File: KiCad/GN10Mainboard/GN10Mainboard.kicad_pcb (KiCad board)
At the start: 4 copper layers, 80 x 60 mm, 129 parts, among them J1 XT30PW-M, J10 USB_C_Receptacle_USB2.0, J13 Conn_01x06, J14 Conn_01x06, J4 Conn_01x04, J5 Conn_01x06, J6 Conn_01x04, J7 Conn_01x04, J8 Conn_01x04, J9 RJ45_Bel_SI-60062-F, SW1 SW_Push, U1 TPS54560DDA, U10 BNO086, U11 FT231XS, U2 3.3V, U4 STM32G474RETx, U5 MCP2562-E-SN, U6 MCP2562-E-SN, U7 MCP2562-E-SN, U8 W5500, Y1 24MHz, Y3 25M, Y6 32.768kHz, Y7 32.768kHz

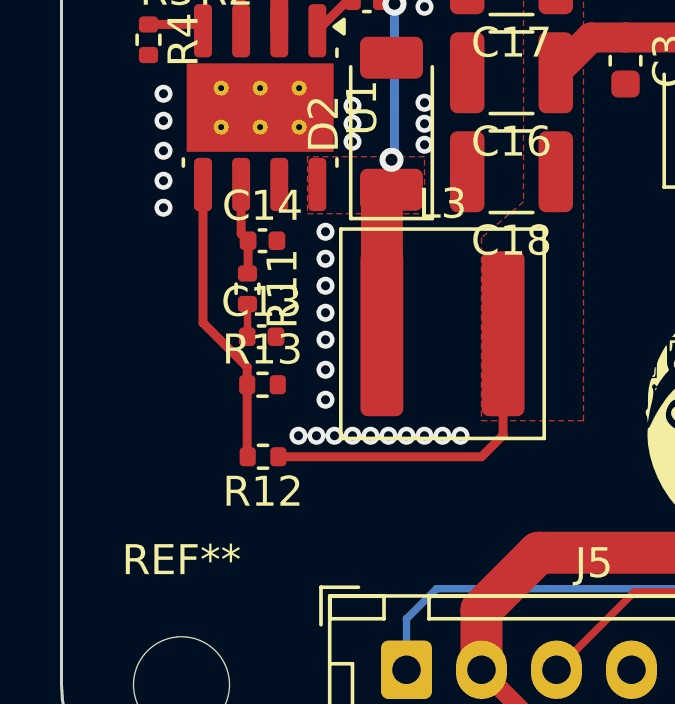
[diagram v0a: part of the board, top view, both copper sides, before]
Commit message: fix:feedback wire
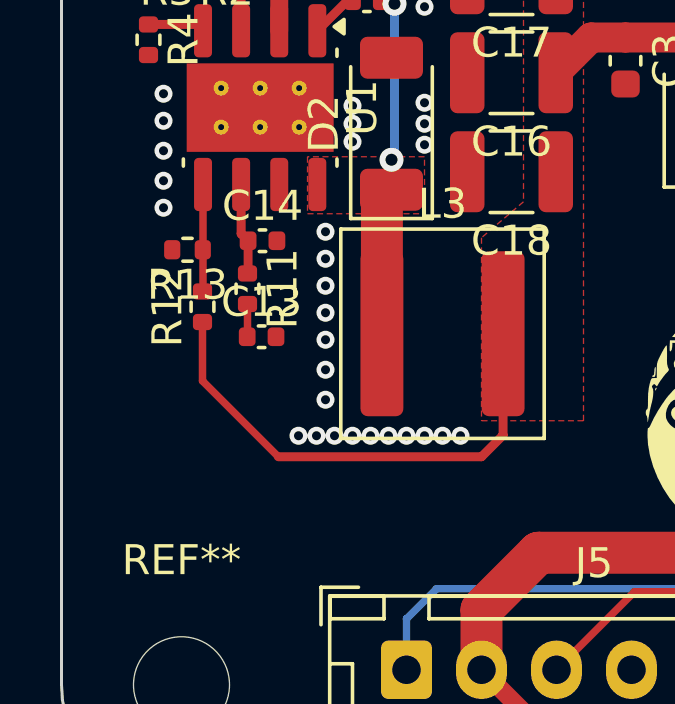
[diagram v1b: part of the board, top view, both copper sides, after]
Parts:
- moved R12 5.39 mm to (134.7, 133.4), turned to 90 degrees
- moved R13 5.15 mm to (134.2, 131.5), turned to 180 degrees
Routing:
- net Net-(U1-FB): track 9.69 -> 3.57 mm
- net +5V: track 98.4 -> 103.9 mm
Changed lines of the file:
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@@
 	(footprint "Resistor_SMD:R_0402_1005Metric"
 		(layer "F.Cu")
-		(at 136.7 136)
+		(at 134.2 131.5 180)
 		(descr "Resistor SMD 0402 (1005 Metric), square (rectangular) end terminal, IPC-7351 nominal, (Body size source: IPC-SM-782 page 72, https://www.pcb-3d.com/wordpress/wp-content/uploads/ipc-sm-782a_amendment_1_and_2.pdf), generated with kicad-footprint-generator")
 		(tags "resistor")
@@
 		(attr smd)
 		(fp_line
-			(start -0.153641 -0.38)
-			(end 0.153641 -0.38)
+			(start -0.153641 0.38)
+			(end 0.153641 0.38)
 			(stroke
 				(width 0.12)
@@
 		)
 		(fp_line
-			(start -0.153641 0.38)
-			(end 0.153641 0.38)
+			(start -0.153641 -0.38)
+			(end 0.153641 -0.38)
 			(stroke
 				(width 0.12)
@@
 		)
 		(fp_line
-			(start -0.93 -0.47)
-			(end 0.93 -0.47)
+			(start 0.93 0.47)
+			(end -0.93 0.47)
 			(stroke
 				(width 0.05)
@@
 		)
 		(fp_line
-			(start -0.93 0.47)
-			(end -0.93 -0.47)
+			(start 0.93 -0.47)
+			(end 0.93 0.47)
 			(stroke
 				(width 0.05)
@@
 		)
 		(fp_line
-			(start 0.93 -0.47)
-			(end 0.93 0.47)
+			(start -0.93 0.47)
+			(end -0.93 -0.47)
 			(stroke
 				(width 0.05)
@@
 		)
 		(fp_line
-			(start 0.93 0.47)
-			(end -0.93 0.47)
+			(start -0.93 -0.47)
+			(end 0.93 -0.47)
 			(stroke
 				(width 0.05)
@@
 		)
 		(fp_line
-			(start -0.525 -0.27)
-			(end 0.525 -0.27)
+			(start 0.525 0.27)
+			(end -0.525 0.27)
 			(stroke
 				(width 0.1)
@@
 		)
 		(fp_line
-			(start -0.525 0.27)
-			(end -0.525 -0.27)
+			(start 0.525 -0.27)
+			(end 0.525 0.27)
 			(stroke
 				(width 0.1)
@@
 		)
 		(fp_line
-			(start 0.525 -0.27)
-			(end 0.525 0.27)
+			(start -0.525 0.27)
+			(end -0.525 -0.27)
 			(stroke
 				(width 0.1)
@@
 		)
 		(fp_line
-			(start 0.525 0.27)
-			(end -0.525 0.27)
+			(start -0.525 -0.27)
+			(end 0.525 -0.27)
 			(stroke
 				(width 0.1)
@@
 		)
 		(pad "1" smd roundrect
-			(at -0.51 0)
+			(at -0.51 0 180)
 			(size 0.54 0.64)
 			(layers "F.Cu" "F.Mask" "F.Paste")
@@
 		)
 		(pad "2" smd roundrect
-			(at 0.51 0)
+			(at 0.51 0 180)
 			(size 0.54 0.64)
 			(layers "F.Cu" "F.Mask" "F.Paste")
@@
 	(footprint "Resistor_SMD:R_0402_1005Metric"
 		(layer "F.Cu")
-		(at 136.7175 138.4 180)
+		(at 134.7 133.4 90)
 		(descr "Resistor SMD 0402 (1005 Metric), square (rectangular) end terminal, IPC-7351 nominal, (Body size source: IPC-SM-782 page 72, https://www.pcb-3d.com/wordpress/wp-content/uploads/ipc-sm-782a_amendment_1_and_2.pdf), generated with kicad-footprint-generator")
 		(tags "resistor")
 		(property "Reference" "R12"
-			(at 0 -1.17 0)
+			(at 0 -1.17 90)
 			(layer "F.SilkS")
 			(effects
@@
 		)
 		(property "Value" "53.6k"
-			(at 0 1.17 0)
+			(at 0 1.17 90)
 			(layer "F.Fab")
 			(effects
@@
 		)
 		(property "Datasheet" "~"
-			(at 0 0 0)
+			(at 0 0 90)
 			(layer "F.Fab")
 			(hide yes)
@@
 		)
 		(property "Description" "Resistor"
-			(at 0 0 0)
+			(at 0 0 90)
 			(layer "F.Fab")
 			(hide yes)
@@
 		(attr smd)
 		(fp_line
-			(start -0.153641 0.38)
-			(end 0.153641 0.38)
+			(start -0.153641 -0.38)
+			(end 0.153641 -0.38)
 			(stroke
 				(width 0.12)
@@
 		)
 		(fp_line
-			(start -0.153641 -0.38)
-			(end 0.153641 -0.38)
+			(start -0.153641 0.38)
+			(end 0.153641 0.38)
 			(stroke
 				(width 0.12)
@@
 		)
 		(fp_line
-			(start 0.93 0.47)
-			(end -0.93 0.47)
+			(start 0.93 -0.47)
+			(end 0.93 0.47)
 			(stroke
 				(width 0.05)
@@
 		)
 		(fp_line
-			(start 0.93 -0.47)
-			(end 0.93 0.47)
+			(start -0.93 -0.47)
+			(end 0.93 -0.47)
 			(stroke
 				(width 0.05)
@@
 		)
 		(fp_line
-			(start -0.93 0.47)
-			(end -0.93 -0.47)
+			(start 0.93 0.47)
+			(end -0.93 0.47)
 			(stroke
 				(width 0.05)
@@
 		)
 		(fp_line
-			(start -0.93 -0.47)
-			(end 0.93 -0.47)
+			(start -0.93 0.47)
+			(end -0.93 -0.47)
 			(stroke
 				(width 0.05)
@@
 		)
 		(fp_line
-			(start 0.525 0.27)
-			(end -0.525 0.27)
+			(start 0.525 -0.27)
+			(end 0.525 0.27)
 			(stroke
 				(width 0.1)
@@
 		)
 		(fp_line
-			(start 0.525 -0.27)
-			(end 0.525 0.27)
+			(start -0.525 -0.27)
+			(end 0.525 -0.27)
 			(stroke
 				(width 0.1)
@@
 		)
 		(fp_line
-			(start -0.525 0.27)
-			(end -0.525 -0.27)
+			(start 0.525 0.27)
+			(end -0.525 0.27)
 			(stroke
 				(width 0.1)
@@
 		)
 		(fp_line
-			(start -0.525 -0.27)
-			(end 0.525 -0.27)
+			(start -0.525 0.27)
+			(end -0.525 -0.27)
 			(stroke
 				(width 0.1)
@@
 		)
 		(fp_text user "${REFERENCE}"
-			(at 0 0 0)
+			(at 0 0 90)
 			(layer "F.Fab")
 			(effects
@@
 		)
 		(pad "1" smd roundrect
-			(at -0.51 0 180)
+			(at -0.51 0 90)
 			(size 0.54 0.64)
 			(layers "F.Cu" "F.Mask" "F.Paste")
@@
 		)
 		(pad "2" smd roundrect
-			(at 0.51 0 180)
+			(at 0.51 0 90)
 			(size 0.54 0.64)
 			(layers "F.Cu" "F.Mask" "F.Paste")
@@
 	)
 	(segment
+		(start 134.7 135.8725)
+		(end 137.2275 138.4)
+		(width 0.25)
+		(layer "F.Cu")
+		(net 4)
+	)
+	(segment
 		(start 144.352651 97.647349)
 		(end 146 96)
@@
 	)
 	(segment
+		(start 134.7 133.91)
+		(end 134.7 135.8725)
+		(width 0.25)
+		(layer "F.Cu")
+		(net 4)
+	)
+	(segment
 		(start 151.554999 111.52)
 		(end 155.1 111.52)
@@
 	(segment
 		(start 134.7175 129.325)
-		(end 134.7175 133.93576)
-		(width 0.3)
-		(layer "F.Cu")
-		(net 77)
-	)
-	(segment
-		(start 136.19 136)
-		(end 136.19 138.3825)
-		(width 0.3)
-		(layer "F.Cu")
-		(net 77)
-	)
-	(segment
-		(start 136.19 135.40826)
-		(end 136.19 136)
-		(width 0.3)
-		(layer "F.Cu")
-		(net 77)
-	)
-	(segment
-		(start 134.7175 133.93576)
-		(end 136.19 135.40826)
-		(width 0.3)
+		(end 134.7175 132.8725)
+		(width 0.25)
 		(layer "F.Cu")
 		(net 77)
 	)
 	(segment
-		(start 136.19 138.3825)
-		(end 136.2075 138.4)
-		(width 0.3)
+		(start 134.7175 132.8725)
+		(end 134.7 132.89)
+		(width 0.25)
 		(layer "F.Cu")
 		(net 77)
